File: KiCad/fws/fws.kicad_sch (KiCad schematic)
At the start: 35 parts, among them J1 USB_C_Receptacle_USB2.0, J2 SM03B-SRSS-TB_LF__SN_, U1 W25Q128JVS, U2 MIC5205-3.3YM5, U3 RP2040, Y1 12MHz

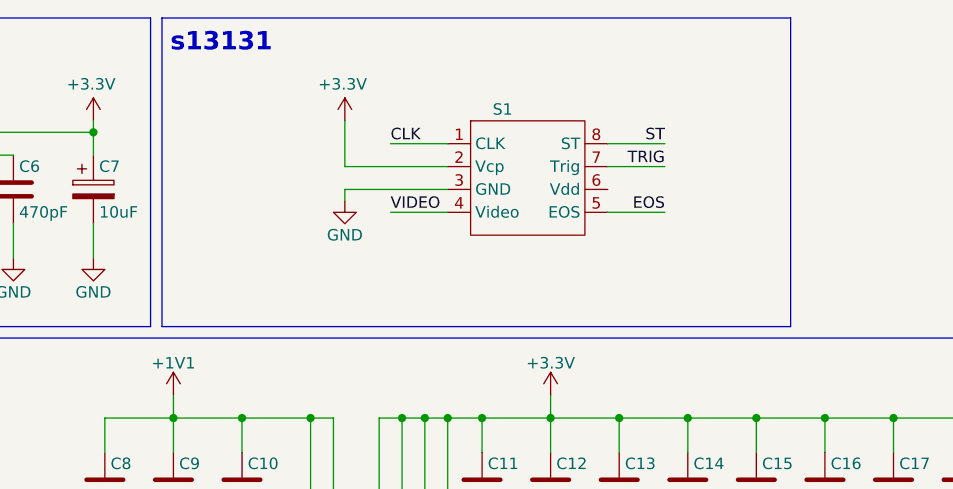
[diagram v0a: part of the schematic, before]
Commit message: Updated schematics.
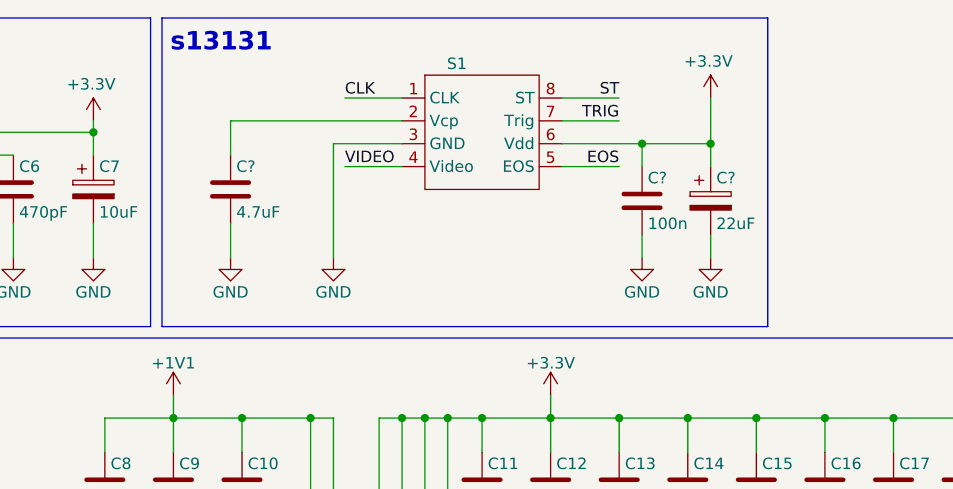
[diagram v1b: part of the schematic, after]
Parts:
- added C?: 4.7uF, Capacitor_SMD:C_0603_1608Metric_Pad1.08x0.95mm_HandSolder, symbol FWS:C
- added C?: 22uF, Capacitor_SMD:C_0603_1608Metric_Pad1.08x0.95mm_HandSolder, symbol FWS:C_Polarized
- added C?: 100n, Capacitor_SMD:C_0603_1608Metric_Pad1.08x0.95mm_HandSolder, symbol FWS:C
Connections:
- net +3.3V: now also S1.6 (Vdd), C?.1, C?.1; no longer S1.2 (Vcp)
- net GND: now also C?.2, C?.2, C?.2
- new net: C?.1, S1.2 (Vcp)
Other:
- moved on the sheet: S1
